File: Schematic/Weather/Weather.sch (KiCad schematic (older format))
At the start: 0 parts

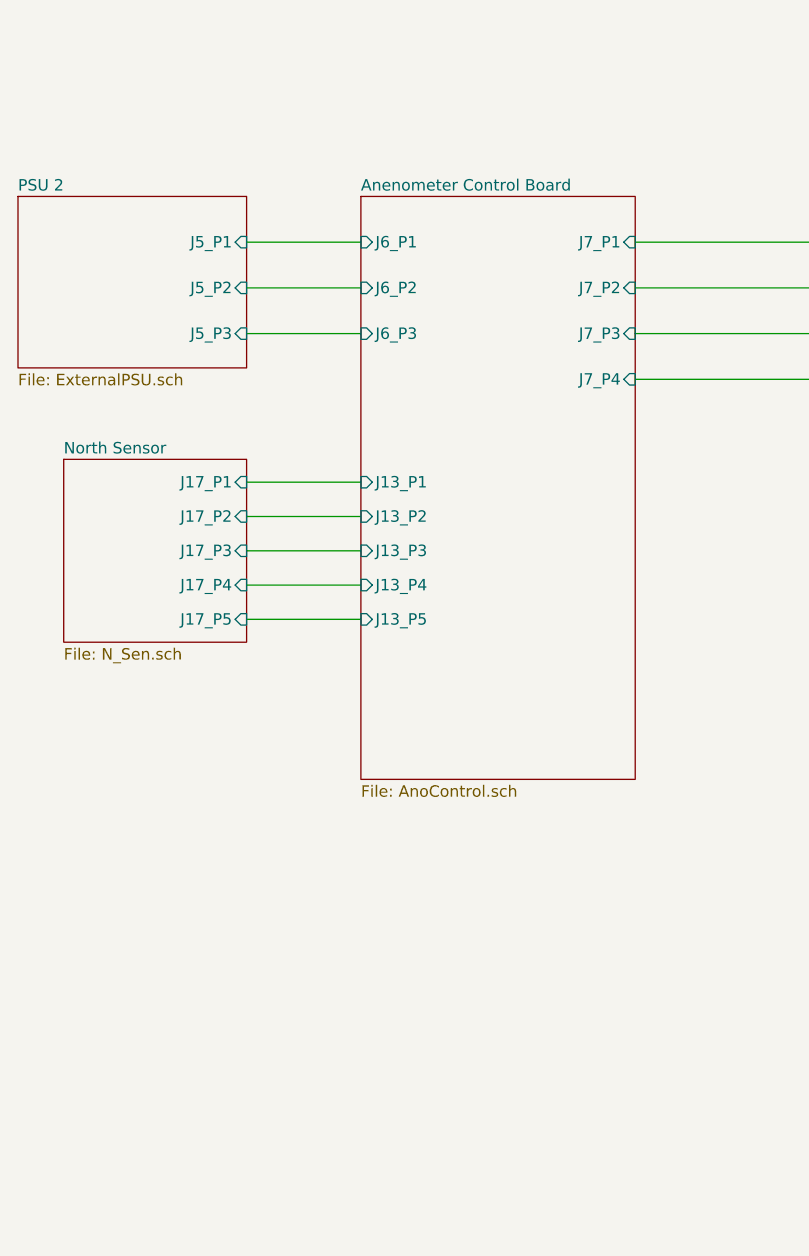
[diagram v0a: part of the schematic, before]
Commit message: more board layouts
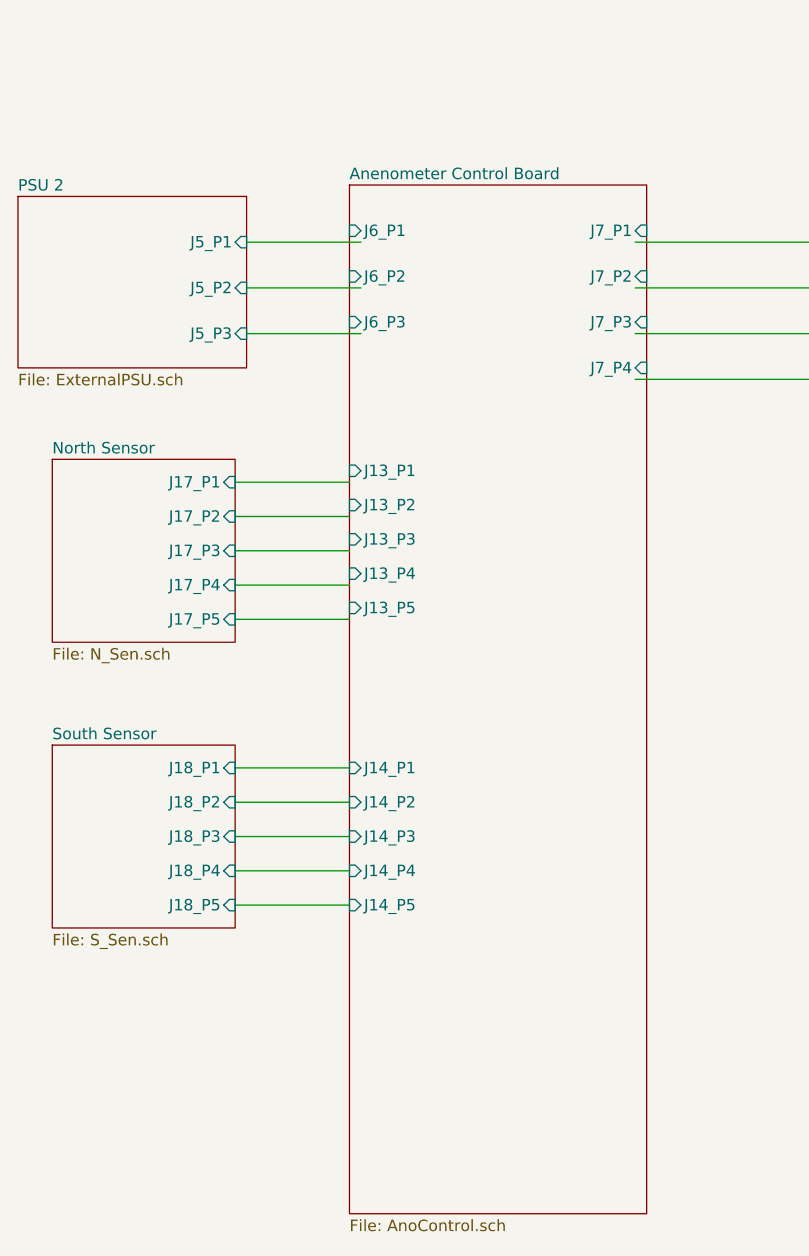
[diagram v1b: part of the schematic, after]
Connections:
- wire segments 26 -> 31
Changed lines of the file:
@@
 $Descr A4 11693 8268
 encoding utf-8
-Sheet 1 10
+Sheet 1 11
 Title ""
 Date ""
@@
 F3 "J5_P2" I R 2500 3400 50
 F4 "J5_P3" I R 2500 3600 50
-$EndSheet
-$Sheet
-S 3000 3000 1200 2550
-U 5C96824E
-F0 "Anenometer Control Board" 50
-F1 "AnoControl.sch" 50
-F2 "J6_P1" I L 3000 3200 50
-F3 "J6_P2" I L 3000 3400 50
-F4 "J6_P3" I L 3000 3600 50
-F5 "J7_P1" I R 4200 3200 50
-F6 "J7_P2" I R 4200 3400 50
-F7 "J7_P3" I R 4200 3600 50
-F8 "J7_P4" I R 4200 3800 50
-F9 "J13_P1" I L 3000 4250 50
-F10 "J13_P2" I L 3000 4400 50
-F11 "J13_P3" I L 3000 4550 50
-F12 "J13_P4" I L 3000 4700 50
-F13 "J13_P5" I L 3000 4850 50
 $EndSheet
 Wire Wire Line
@@
 	6500 4600 7500 4600
 Wire Wire Line
-	2500 4250 3000 4250
+	2450 4250 2950 4250
 Wire Wire Line
-	2500 4550 3000 4550
+	2450 4550 2950 4550
 Wire Wire Line
-	2500 4400 3000 4400
+	2450 4400 2950 4400
 Wire Wire Line
-	2500 4700 3000 4700
+	2450 4700 2950 4700
 Wire Wire Line
-	2500 4850 3000 4850
+	2450 4850 2950 4850
 $Sheet
-S 1700 4150 800  800
+S 1650 4150 800  800
 U 5C952539
 F0 "North Sensor" 50
 F1 "N_Sen.sch" 50
-F2 "J17_P1" I R 2500 4250 50
-F3 "J17_P2" I R 2500 4400 50
-F4 "J17_P3" I R 2500 4550 50
-F5 "J17_P4" I R 2500 4700 50
-F6 "J17_P5" I R 2500 4850 50
+F2 "J17_P1" I R 2450 4250 50
+F3 "J17_P2" I R 2450 4400 50
+F4 "J17_P3" I R 2450 4550 50
+F5 "J17_P4" I R 2450 4700 50
+F6 "J17_P5" I R 2450 4850 50
 $EndSheet
+$Sheet
+S 1650 5400 800  800
+U 5C9F4D88
+F0 "South Sensor" 50
+F1 "S_Sen.sch" 50
+F2 "J18_P1" I R 2450 5500 50
+F3 "J18_P2" I R 2450 5650 50
+F4 "J18_P3" I R 2450 5800 50
+F5 "J18_P4" I R 2450 5950 50
+F6 "J18_P5" I R 2450 6100 50
+$EndSheet
+$Sheet
+S 2950 2950 1300 4500
+U 5C96824E
+F0 "Anenometer Control Board" 50
+F1 "AnoControl.sch" 50
+F2 "J6_P1" I L 2950 3150 50
+F3 "J6_P2" I L 2950 3350 50
+F4 "J6_P3" I L 2950 3550 50
+F5 "J7_P1" I R 4250 3150 50
+F6 "J7_P2" I R 4250 3350 50
+F7 "J7_P3" I R 4250 3550 50
+F8 "J7_P4" I R 4250 3750 50
+F9 "J13_P1" I L 2950 4200 50
+F10 "J13_P2" I L 2950 4350 50
+F11 "J13_P3" I L 2950 4500 50
+F12 "J13_P4" I L 2950 4650 50
+F13 "J13_P5" I L 2950 4800 50
+F14 "J14_P1" I L 2950 5500 50
+F15 "J14_P2" I L 2950 5650 50
+F16 "J14_P3" I L 2950 5800 50
+F17 "J14_P4" I L 2950 5950 50
+F18 "J14_P5" I L 2950 6100 50
+$EndSheet
+Wire Wire Line
+	2450 5500 2950 5500
+Wire Wire Line
+	2450 5650 2950 5650
+Wire Wire Line
+	2450 5800 2950 5800
+Wire Wire Line
+	2450 5950 2950 5950
+Wire Wire Line
+	2450 6100 2950 6100
 $EndSCHEMATC
